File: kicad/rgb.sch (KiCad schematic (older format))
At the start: 25 parts, among them J1 1935776, J2 102-6164-ND, J3 102-6164-ND, J4 Conn_01x04, J5 Conn_01x02, Q1 DMG9926USD, Q2 DMG9926USD, Q3 DMG9926USD, Q4 DMG9926USD, SW1 450-1642-ND, SW2 PEC12R-4220F-N0024, SW3 PEC12R-4220F-N0024, SW4 PEC12R-4220F-N0024, SW5 PEC12R-4220F-N0024, SW6 450-1642-ND, U1 ATtiny416-SNR, U2 576-1256-2-ND

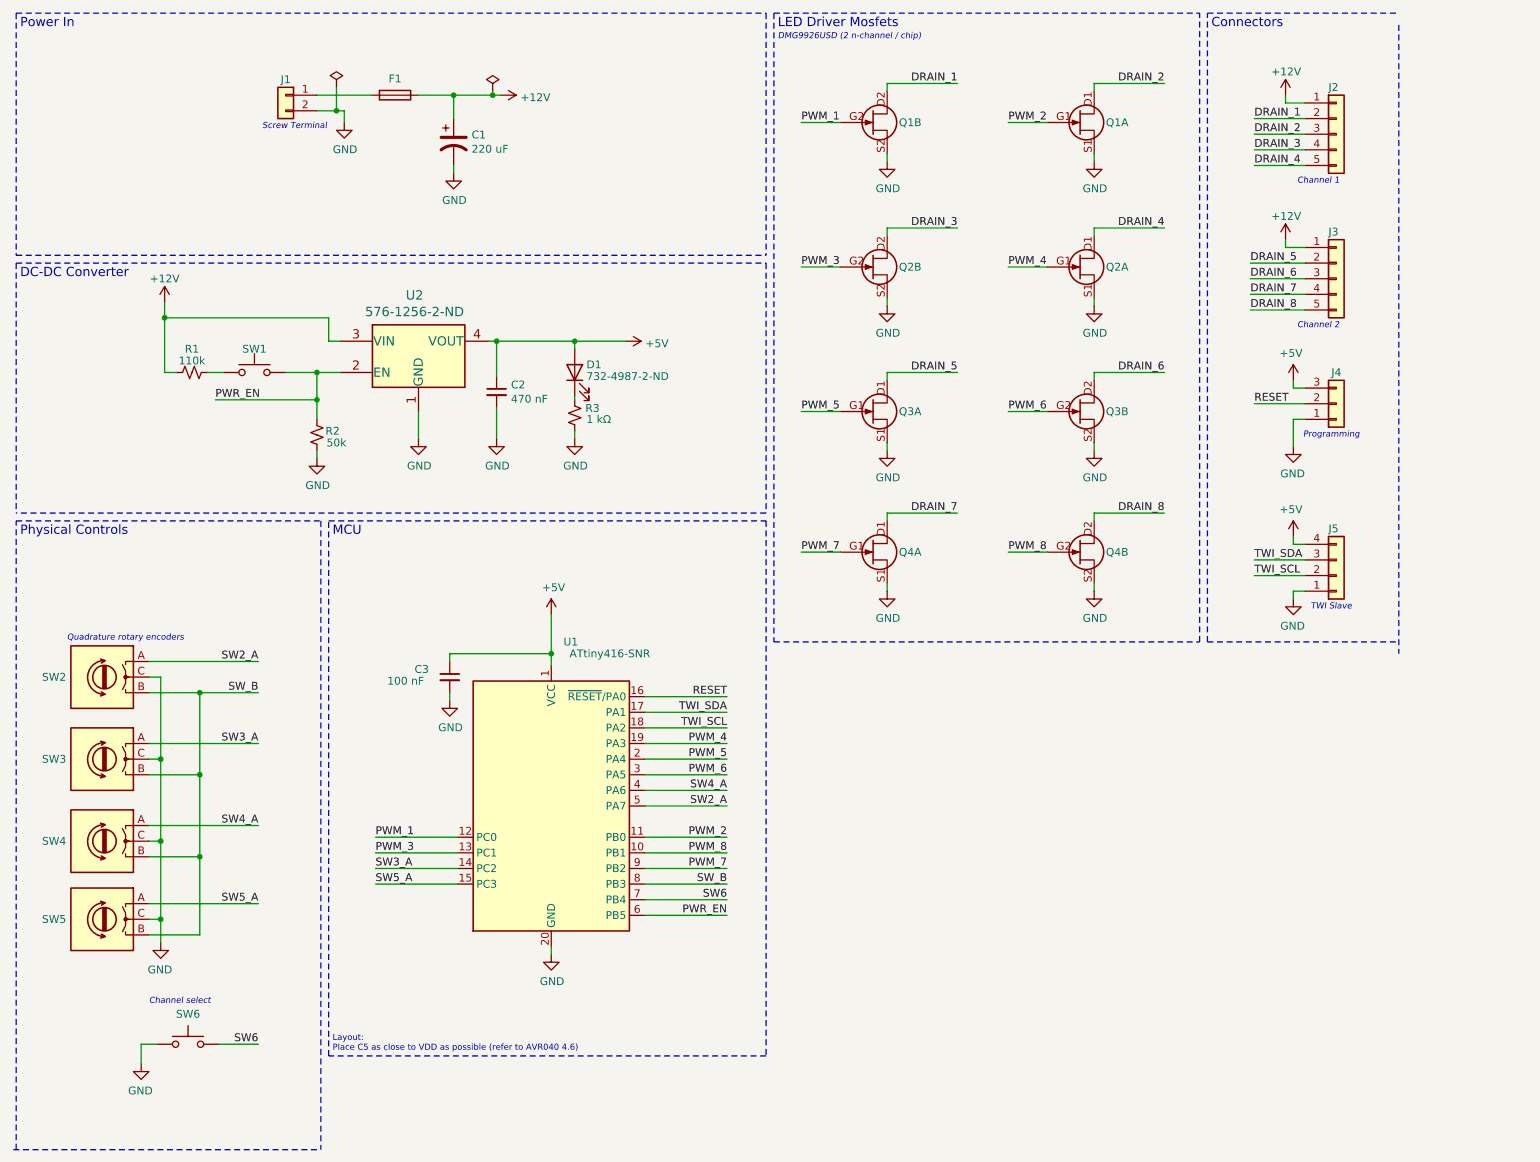
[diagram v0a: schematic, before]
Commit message: layout done
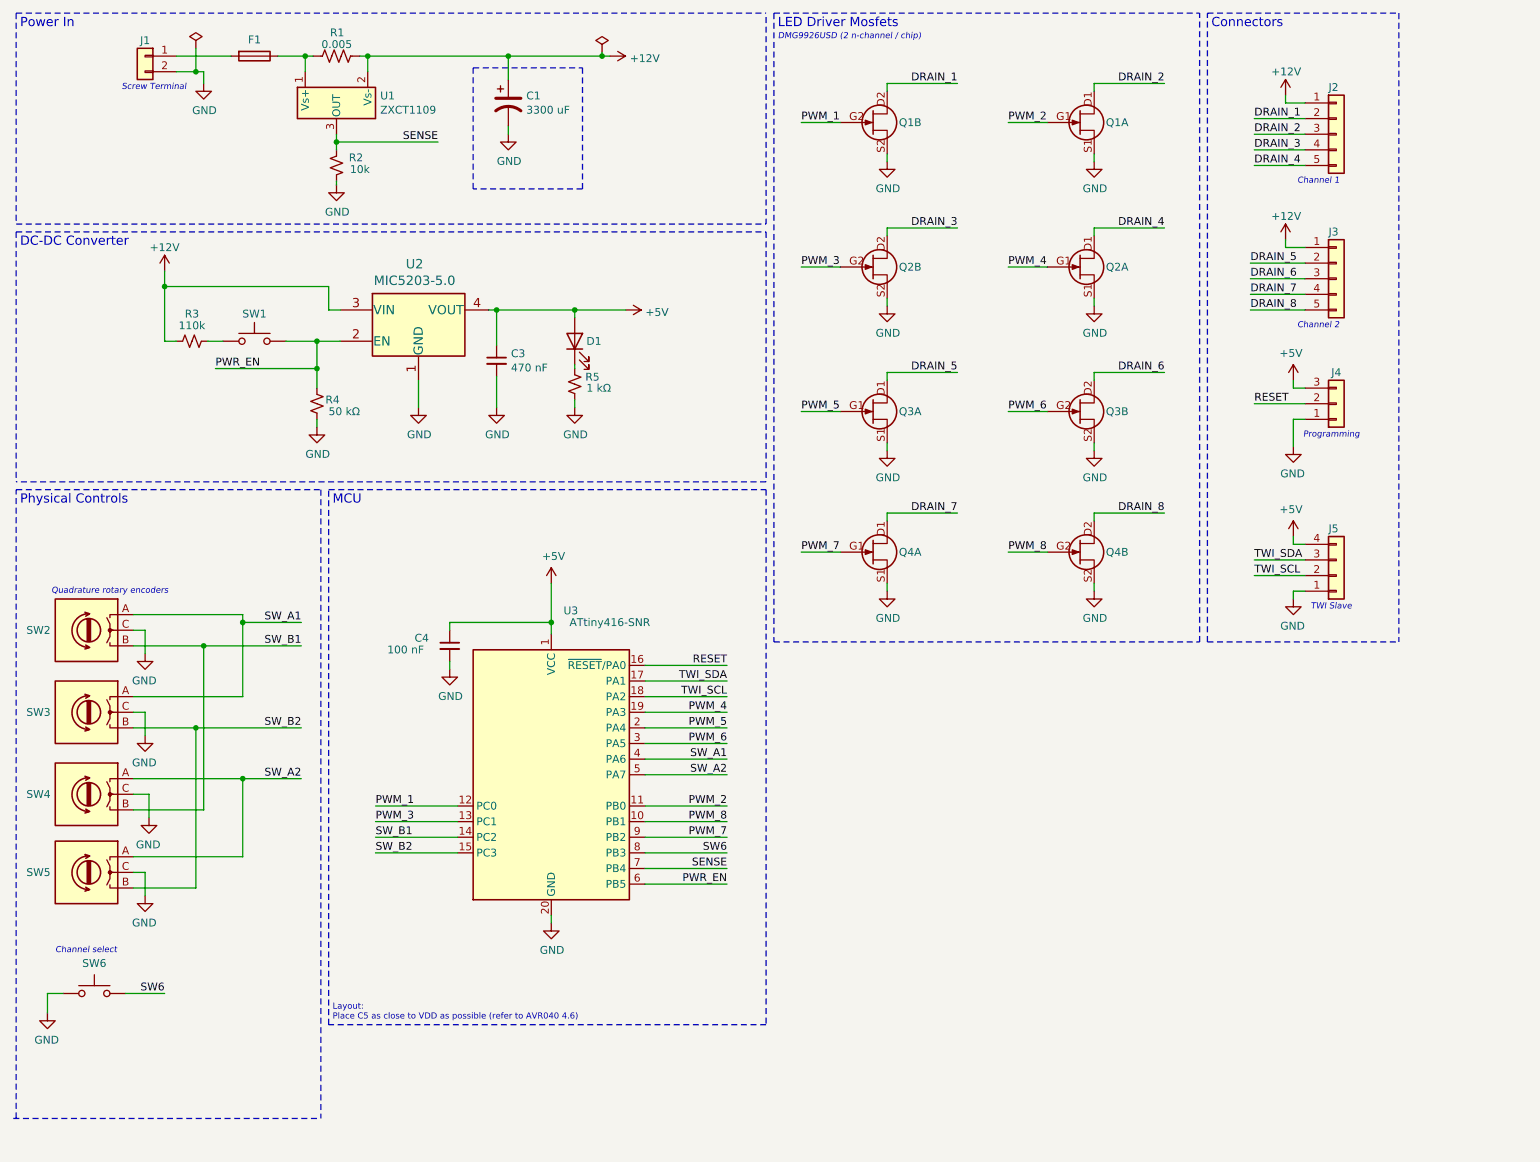
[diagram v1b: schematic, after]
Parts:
- added R1: 0.005, Resistor_SMD:R_1020_2550Metric_Pad1.33x5.20mm_HandSolder, symbol Device:R_US
- added R2: 10k, Resistor_SMD:R_0805_2012Metric_Pad1.20x1.40mm_HandSolder, symbol Device:R_Small_US
- added U1: ZXCT1109, Package_TO_SOT_SMD:SOT-23, symbol Amplifier_Current:ZXCT1107
- C1: value 220 uF -> 3300 uF; footprint Capacitor_SMD:CP_Elec_6.3x7.7 -> Capacitor_THT:CP_Radial_D12.5mm_P5.00mm
- R4: renamed from R2; value 50k -> 50 kΩ
- U2: value 576-1256-2-ND -> MIC5203-5.0
- renumbered C2 to C3, C3 to C4, R1 to R3, R3 to R5, U1 to U3
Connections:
- net +12V: now also R1.2, U1.2 (Vs-); no longer F1.1
- net GND: now also R2.2
- net SW6: now also U3.8 (PB3); no longer U3.7 (PB4)
- net SW2_A renamed SW_A1
- net SW_A1: now also SW3.A, U3.4 (PA6); no longer U3.5 (PA7)
- net SW3_A renamed SW_B1
- net SW_B1: now also SW2.B, SW4.B; no longer SW3.A
- net SW4_A renamed SW_A2
- net SW_A2: now also SW5.A, U3.5 (PA7); no longer U3.4 (PA6)
- net SW5_A renamed SW_B2
- net SW_B2: now also SW3.B, SW5.B; no longer SW5.A
- removed net SW_B: SW2.B, SW3.B, SW4.B, SW5.B, U3.8 (PB3)
- new net: F1.1, R1.1, U1.1 (Vs+)
- new net SENSE: R2.1, U1.3 (OUT), U3.7 (PB4)
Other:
- moved on the sheet: C3, C4, D1, F1, J1, R3, R4, R5, SW1, SW2, SW3, SW4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

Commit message: rev0
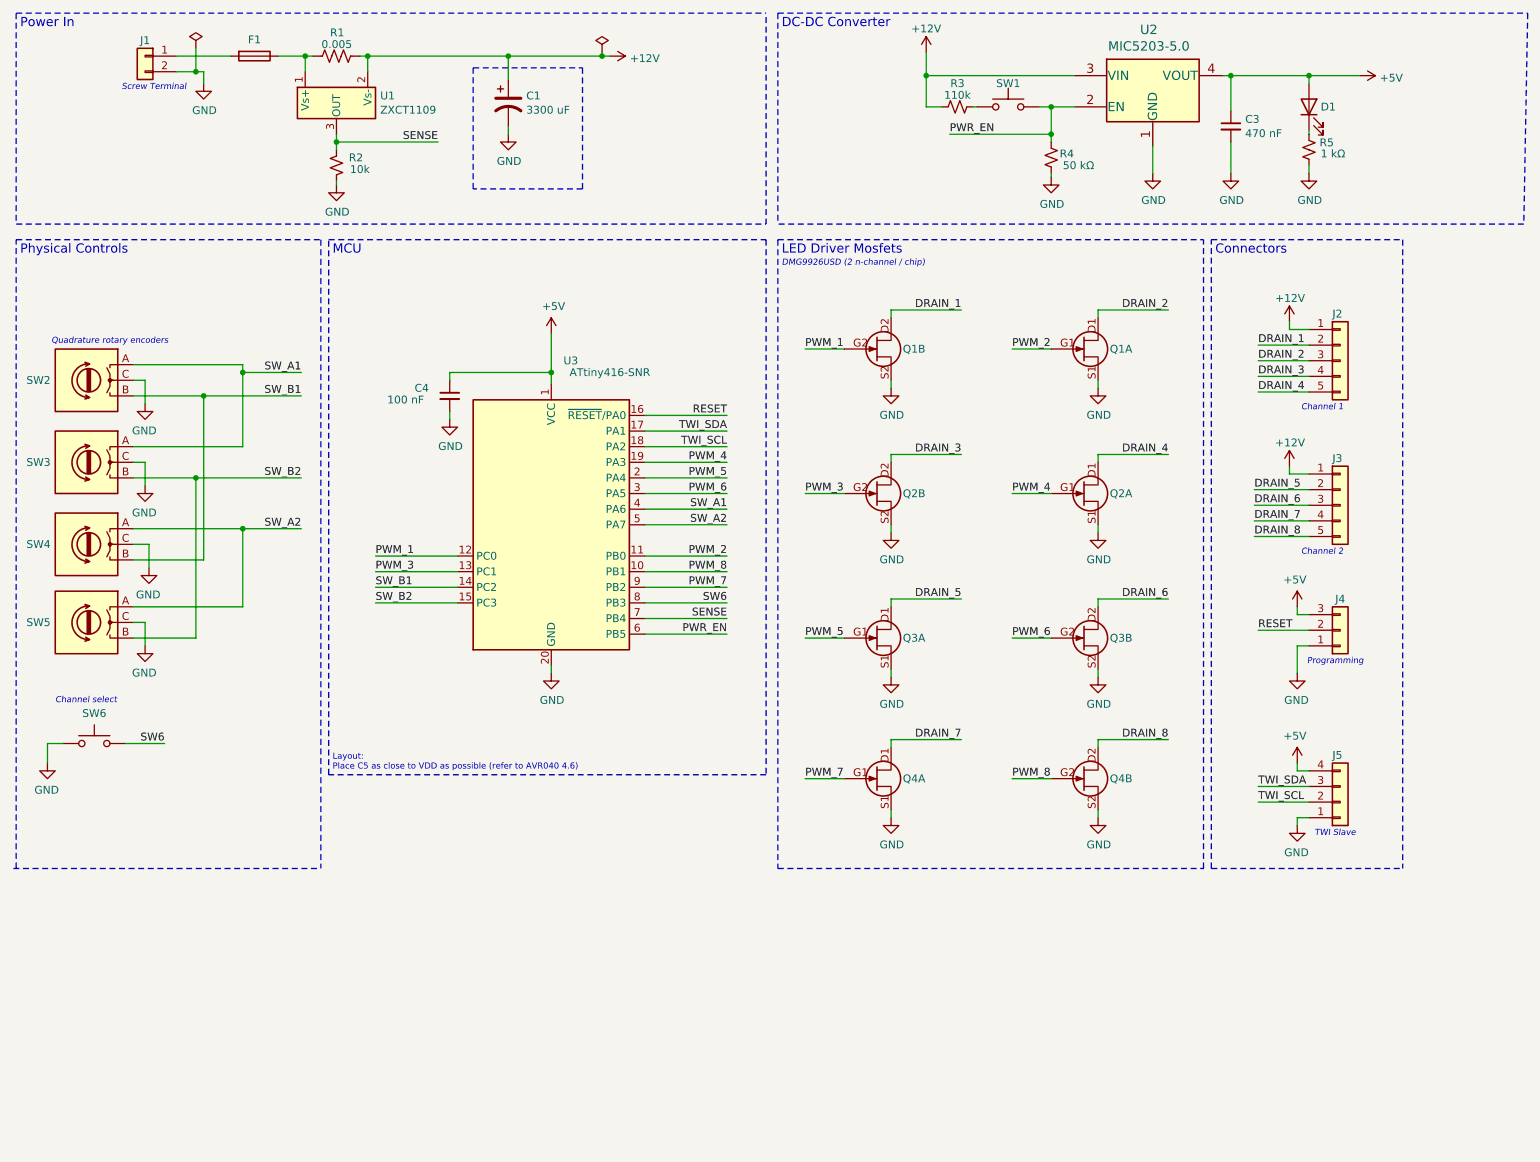
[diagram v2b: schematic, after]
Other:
- moved on the sheet: C3, C4, D1, J2, J3, J4, J5, Q1A, Q1B, Q2A, Q2B, Q3A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

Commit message: minor changes
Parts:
- U2: symbol MIC5203:MIC5203-5.0YM4-TR -> rgb-rescue:MIC5203-5.0YM4-TR-MIC5203
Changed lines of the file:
@@
 $EndComp
 $Comp
-L MIC5203:MIC5203-5.0YM4-TR U2
+L rgb-rescue:MIC5203-5.0YM4-TR-MIC5203 U2
 U 1 1 5FEE6BDA
 P 7825 1250
